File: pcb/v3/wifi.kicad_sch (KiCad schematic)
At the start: 12 parts, among them U11 TXS0102DCU, U12 TXS0102DCU, U8 M8800DU6

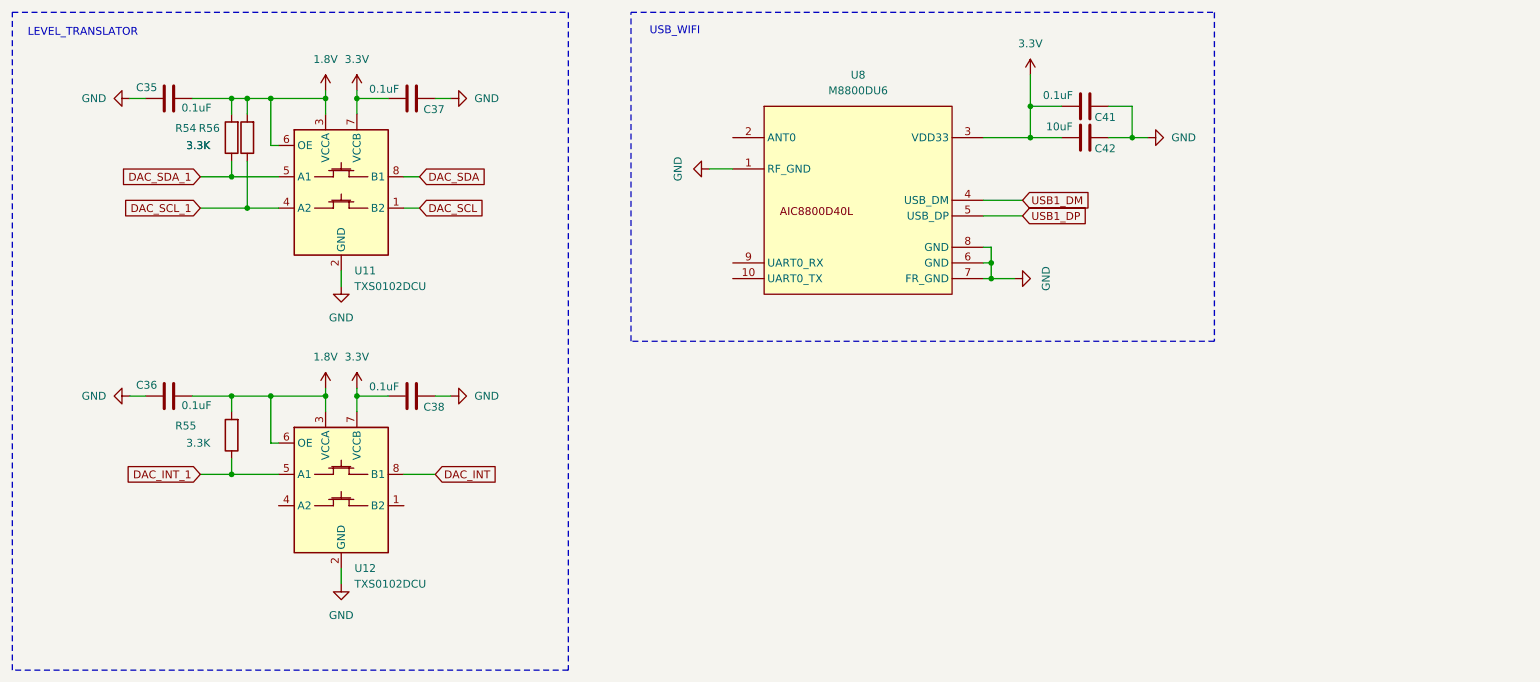
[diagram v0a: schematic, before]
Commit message: up
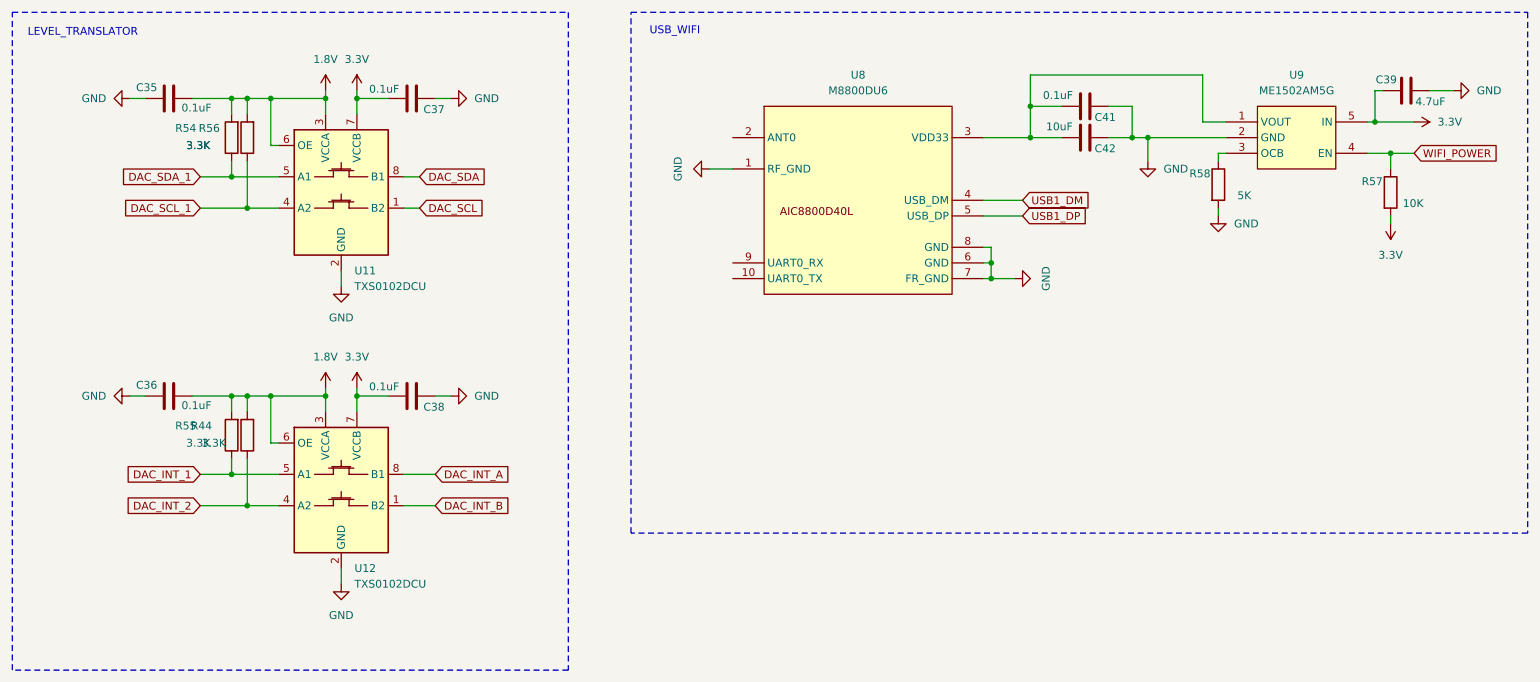
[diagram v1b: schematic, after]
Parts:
- added C39: 4.7uF, Capacitor_SMD:C_0402_1005Metric_Pad0.74x0.62mm_HandSolder, symbol Device:C
- added R44: 3.3K, Capacitor_SMD:C_0402_1005Metric_Pad0.74x0.62mm_HandSolder, symbol Device:R
- added R57: 10K, Capacitor_SMD:C_0402_1005Metric_Pad0.74x0.62mm_HandSolder, symbol Device:R
- added R58: 5K, Capacitor_SMD:C_0402_1005Metric_Pad0.74x0.62mm_HandSolder, symbol Device:R
- added U9: ME1502AM5G, Package_TO_SOT_SMD:SOT-23-5, symbol coloryr:ETA6280S2F
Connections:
- net 1.8V: now also R44.2
- net 3.3V: now also C39.1, R57.2, U9.5 (IN); no longer C41.2, C42.2, U8.3 (VDD33)
- net GND: now also C39.2, R58.2, U9.2 (GND)
- net DAC_INT_B: now reaches U12.1 (B2)
- net DAC_INT_2: now reaches U12.4 (A2)
- net DAC_INT_2: now also R44.1
- net DAC_INT renamed DAC_INT_A
- new net: C41.2, C42.2, U8.3 (VDD33), U9.1 (VOUT)
- new net: R58.1, U9.3 (OCB)
- new net WIFI_POWER: R57.1, U9.4 (EN)
